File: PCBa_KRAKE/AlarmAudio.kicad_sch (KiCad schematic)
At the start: 15 parts, among them J1 DFPlayermini, J601 1X2P 1.25 mm Header, J602 0.100_2Pin, J603 2mm_2Pin

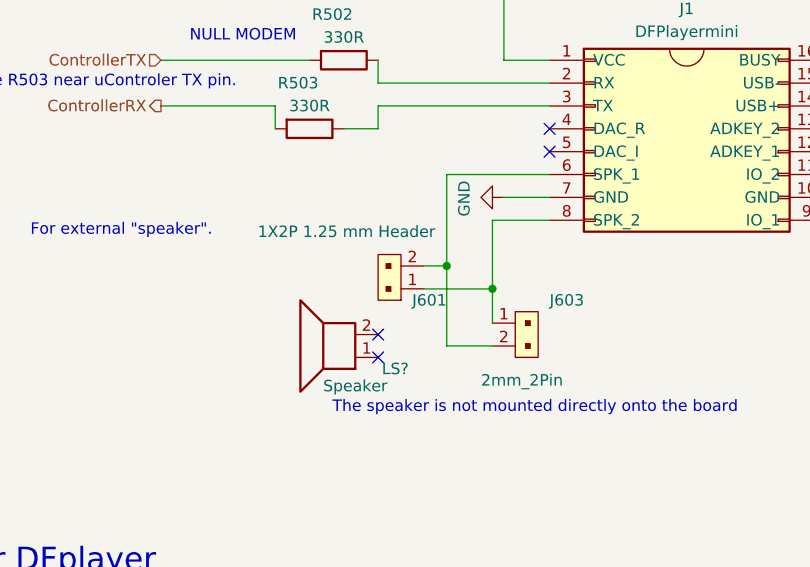
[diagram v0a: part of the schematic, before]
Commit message: AlarmAudio.kicad_sch, Restoring older version of schematic after accidently making Eev2 changes to it.
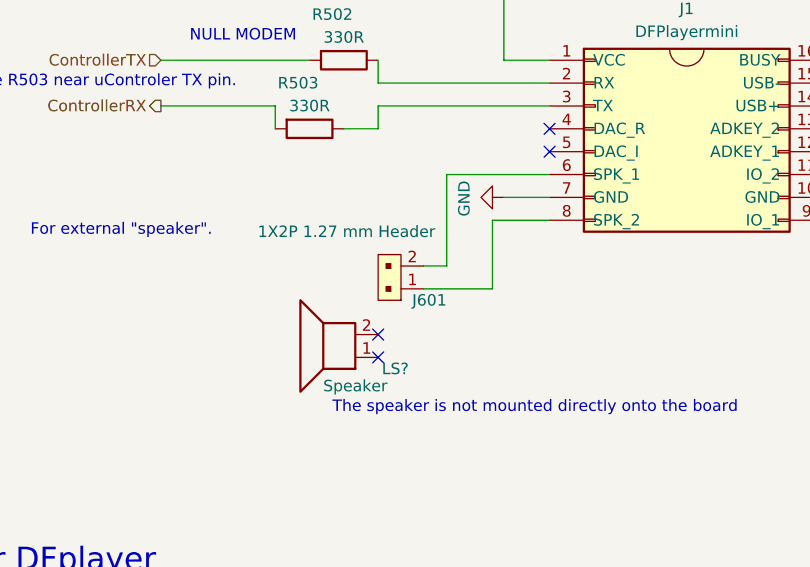
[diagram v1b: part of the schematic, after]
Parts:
- removed J603: 2mm_2Pin, Connector_JST:JST_PH_B2B-PH-K_1x02_P2.00mm_Vertical, symbol GPAD_SCH_LIB:22-23-2021
- J601: value 1X2P 1.25 mm Header -> 1X2P 1.27 mm Header; footprint Connector_Molex:Molex_PicoBlade_53047-0210_1x02_P1.25mm_Vertical -> Connector_PinHeader_1.27mm:PinHeader_1x02_P1.27mm_Vertical; Distributor 1 PN C114130 -> C7496728; MPN 530470210 -> PZ150V-02P; Manufacturer MOLEX -> XFCN
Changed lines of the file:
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@@
   (junction (at 66.04 81.28) (diameter 0) (color 0 0 0 0)
-  )
-  (junction (at 182.88 128.27) (diameter 0) (color 0 0 0 0)
-  )
-  (junction (at 187.96 130.81) (diameter 0) (color 0 0 0 0)
   )
   (junction (at 78.74 81.28) (diameter 0) (color 0 0 0 0)
@@
     (stroke (width 0) (type default))
   )
-  (wire (pts (xy 187.96 137.16) (xy 182.88 137.16))
-    (stroke (width 0) (type default))
-  )
-  (wire (pts (xy 182.88 128.27) (xy 182.88 137.16))
-    (stroke (width 0) (type default))
-  )
   (wire (pts (xy 163.83 110.49) (xy 151.13 110.49))
     (stroke (width 0) (type default))
@@
     (stroke (width 0) (type default))
   )
-  (wire (pts (xy 182.88 118.11) (xy 182.88 128.27))
-    (stroke (width 0) (type default))
-  )
   (wire (pts (xy 44.45 81.28) (xy 44.45 77.47))
     (stroke (width 0) (type default))
@@
     (stroke (width 0) (type default))
   )
+  (wire (pts (xy 182.88 128.27) (xy 182.88 118.11))
+    (stroke (width 0) (type default))
+  )
   (wire (pts (xy 213.36 67.31) (xy 217.17 67.31))
     (stroke (width 0) (type default))
@@
   )
   (wire (pts (xy 187.96 123.19) (xy 194.31 123.19))
-    (stroke (width 0) (type default))
-  )
-  (wire (pts (xy 187.96 130.81) (xy 187.96 134.62))
     (stroke (width 0) (type default))
   )
@@
       (effects (font (size 1.27 1.27)) (justify right))
     )
-    (property "Value" "1X2P 1.25 mm Header" (at 181.61 124.46 90)
+    (property "Value" "1X2P 1.27 mm Header" (at 181.61 124.46 90)
       (effects (font (size 1.27 1.27)) (justify right))
     )
-    (property "Footprint" "Connector_Molex:Molex_PicoBlade_53047-0210_1x02_P1.25mm_Vertical" (at 182.88 125.73 0)
+    (property "Footprint" "Connector_PinHeader_1.27mm:PinHeader_1x02_P1.27mm_Vertical" (at 182.88 125.73 0)
       (effects (font (size 1.524 1.524)) (justify left) hide)
     )
@@
       (effects (font (size 1.524 1.524)) (justify left) hide)
     )
-    (property "MPN" "530470210" (at 190.5 125.73 0)
+    (property "MPN" "PZ150V-02P" (at 190.5 125.73 0)
       (effects (font (size 1.524 1.524)) (justify left) hide)
     )
@@
       (effects (font (size 1.524 1.524)) (justify left) hide)
     )
-    (property "Description" "1.25mm 1x2P 2 2P 3.2mm 4.25mm 4.2mm PA Phosphor Bronze PicoBlade(MX 1.25) " (at 203.2 125.73 0)
-      (effects (font (size 1.524 1.524)) (justify left) hide)
-    )
-    (property "Manufacturer" "MOLEX" (at 205.74 125.73 0)
+    (property "Description" "Direct Insert 2P 1.5mm Single Row 1x2P Plugin,P=1.5mm Pin Headers ROHS" (at 203.2 125.73 0)
+      (effects (font (size 1.524 1.524)) (justify left) hide)
+    )
+    (property "Manufacturer" "XFCN" (at 205.74 125.73 0)
       (effects (font (size 1.524 1.524)) (justify left) hide)
     )
@@
       (effects (font (size 1.27 1.27)) hide)
     )
-    (property "Distributor 1 PN" "C114130" (at 177.8 130.81 0)
+    (property "Distributor 1 PN" "C7496728" (at 177.8 130.81 0)
       (effects (font (size 1.27 1.27)) hide)
     )
@@
         )
       )
-    )
-  )
-  (symbol (lib_id "GPAD_SCH_LIB:22-23-2021") (at 190.5 134.62 90) (mirror x) (unit 1)
-    (in_bom yes) (on_board yes) (dnp no)
-    (property "Reference" "J603" (at 194.31 132.08 90)
-      (effects (font (size 1.27 1.27)) (justify right))
-    )
-    (property "Value" "2mm_2Pin" (at 186.69 140.97 90)
-      (effects (font (size 1.27 1.27)) (justify right))
-    )
-    (property "Footprint" "Connector_JST:JST_PH_B2B-PH-K_1x02_P2.00mm_Vertical" (at 185.42 139.7 0)
-      (effects (font (size 1.524 1.524)) (justify left) hide)
-    )
-    (property "Datasheet" "https://jlcpcb.com/api/file/downloadByFileSystemAccessId/8588889744620572672" (at 182.88 139.7 0)
-      (effects (font (size 1.524 1.524)) (justify left) hide)
-    )
-    (property "Digi-Key_PN" "B2B-PH-K-S" (at 180.34 139.7 0)
-      (effects (font (size 1.524 1.524)) (justify left) hide)
-    )
-    (property "MPN" "B2B-PH-K-S(LF)(SN)" (at 177.8 139.7 0)
-      (effects (font (size 1.524 1.524)) (justify left) hide)
-    )
-    (property "Category" "Connectors, Interconnects" (at 175.26 139.7 0)
-      (effects (font (size 1.524 1.524)) (justify left) hide)
-    )
-    (property "Description" "HEADER VERT 2POS 2MM" (at 165.1 139.7 0)
-      (effects (font (size 1.524 1.524)) (justify left) hide)
-    )
-    (property "Manufacturer" "JST" (at 162.56 139.7 0)
-      (effects (font (size 1.524 1.524)) (justify left) hide)
-    )
-    (property "Status" "Active" (at 160.02 139.7 0)
-      (effects (font (size 1.524 1.524)) (justify left) hide)
-    )
-    (property "Cost" "0.0306" (at 190.5 134.62 0)
-      (effects (font (size 1.27 1.27)) hide)
-    )
-    (property "Distributor 1" "JLCPCB" (at 190.5 134.62 0)
-      (effects (font (size 1.27 1.27)) hide)
-    )
-    (property "Distributor 1 PN" "C131337" (at 190.5 134.62 0)
-      (effects (font (size 1.27 1.27)) hide)
-    )
-    (property "MPN 2" "" (at 190.5 134.62 0)
-      (effects (font (size 1.27 1.27)) hide)
-    )
-    (property "Manufacturer 2" "" (at 190.5 134.62 0)
-      (effects (font (size 1.27 1.27)) hide)
-    )
-    (pin "1")
-    (pin "2")
-    (instances
-      (project "PCBa_KRAKE"
-        (path "/412a327d-1ee3-473e-bc00-1545004b7edf/00000000-0000-0000-0000-000062dd8e5f"
-          (reference "J603") (unit 1)
-        )
-      )
